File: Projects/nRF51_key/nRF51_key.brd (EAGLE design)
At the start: 58.4 x 12 mm, 23 parts, among them IC1 FT230XQ, J1 47571-0001, X1 USBPCB

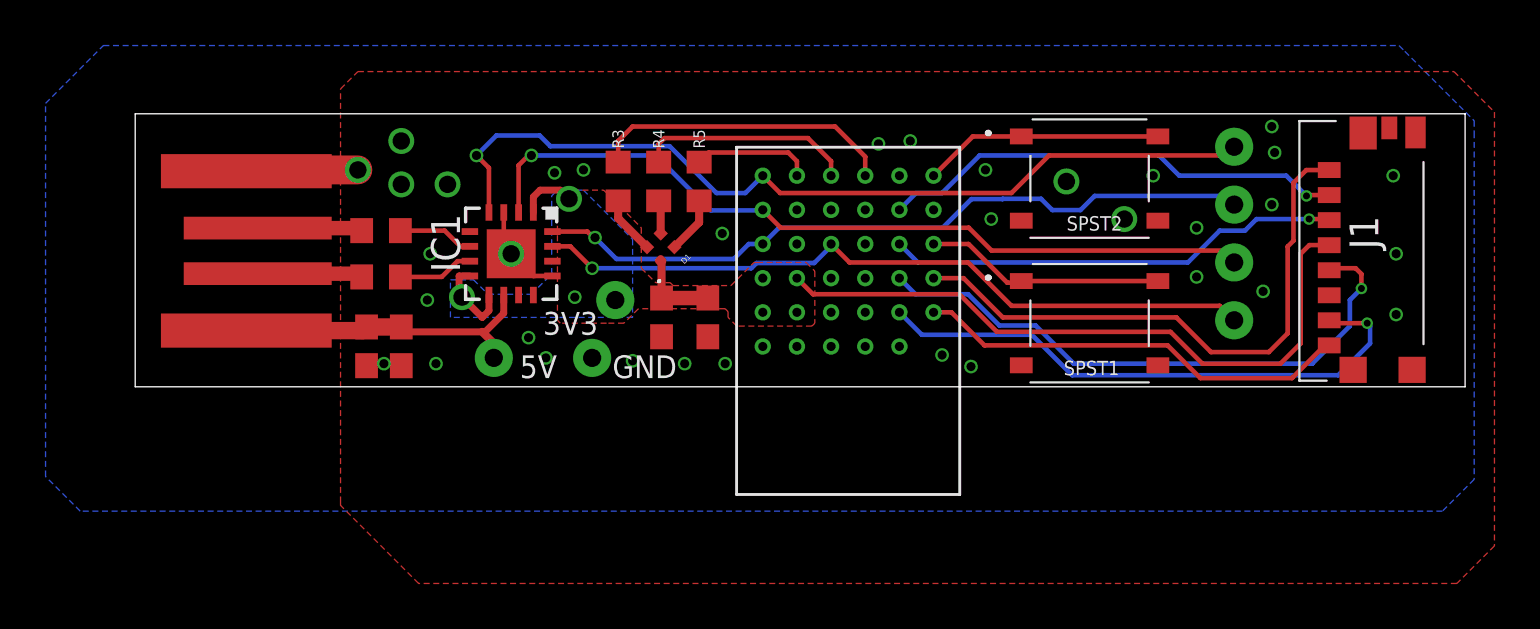
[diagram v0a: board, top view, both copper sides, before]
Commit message: Order @ Boktech
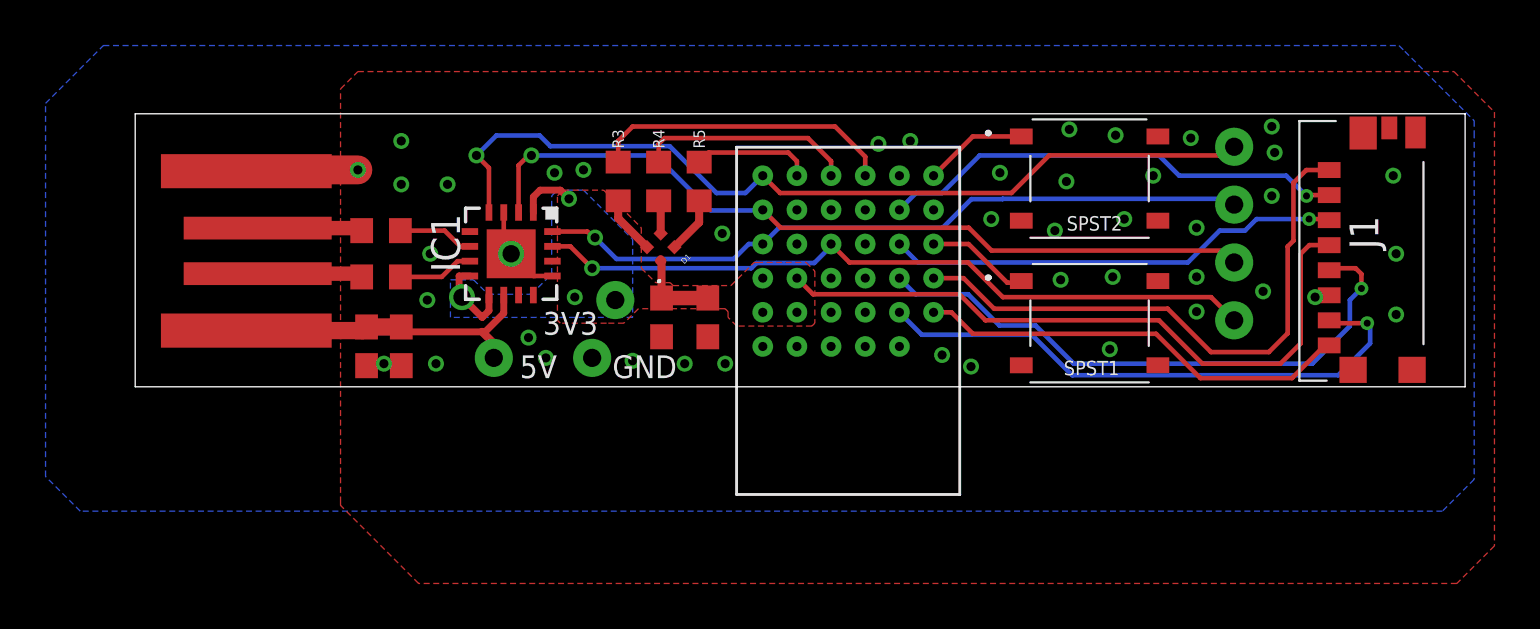
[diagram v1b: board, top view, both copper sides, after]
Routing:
- net BTN2: track 10.6 -> 4.56 mm
- net BTN1: track 10.6 -> 4.58 mm
- net GND: track 9.09 -> 9.74 mm, vias 35 -> 44
- net !RTS: track 32.3 -> 31.7 mm
